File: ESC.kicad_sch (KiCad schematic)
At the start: 23 parts, among them IC1 DRV8302DCA, J1 Prog, J2 Conn_01x01, J3 Conn_01x01, J4 Conn_01x01, J5 Conn_ALIM_MOTOR, J6 Conn_ALIM_AUX, Q1 2N7002, U1 ATmega328P-AU_full, Y1 CSTCE

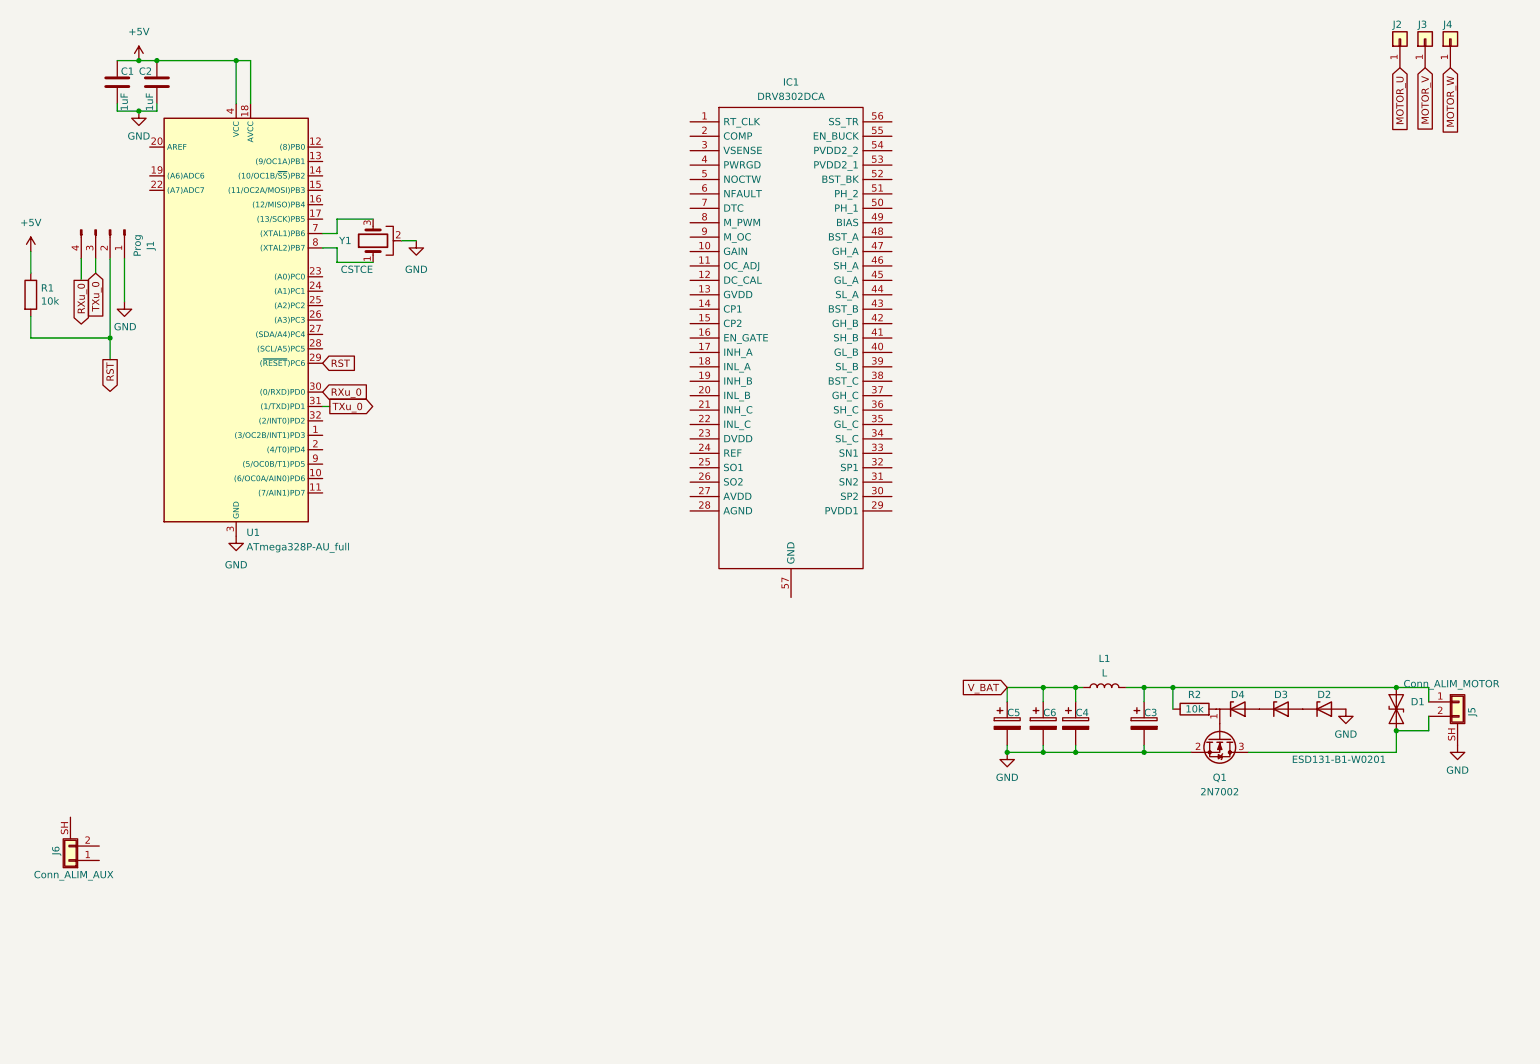
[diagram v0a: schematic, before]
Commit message: aa
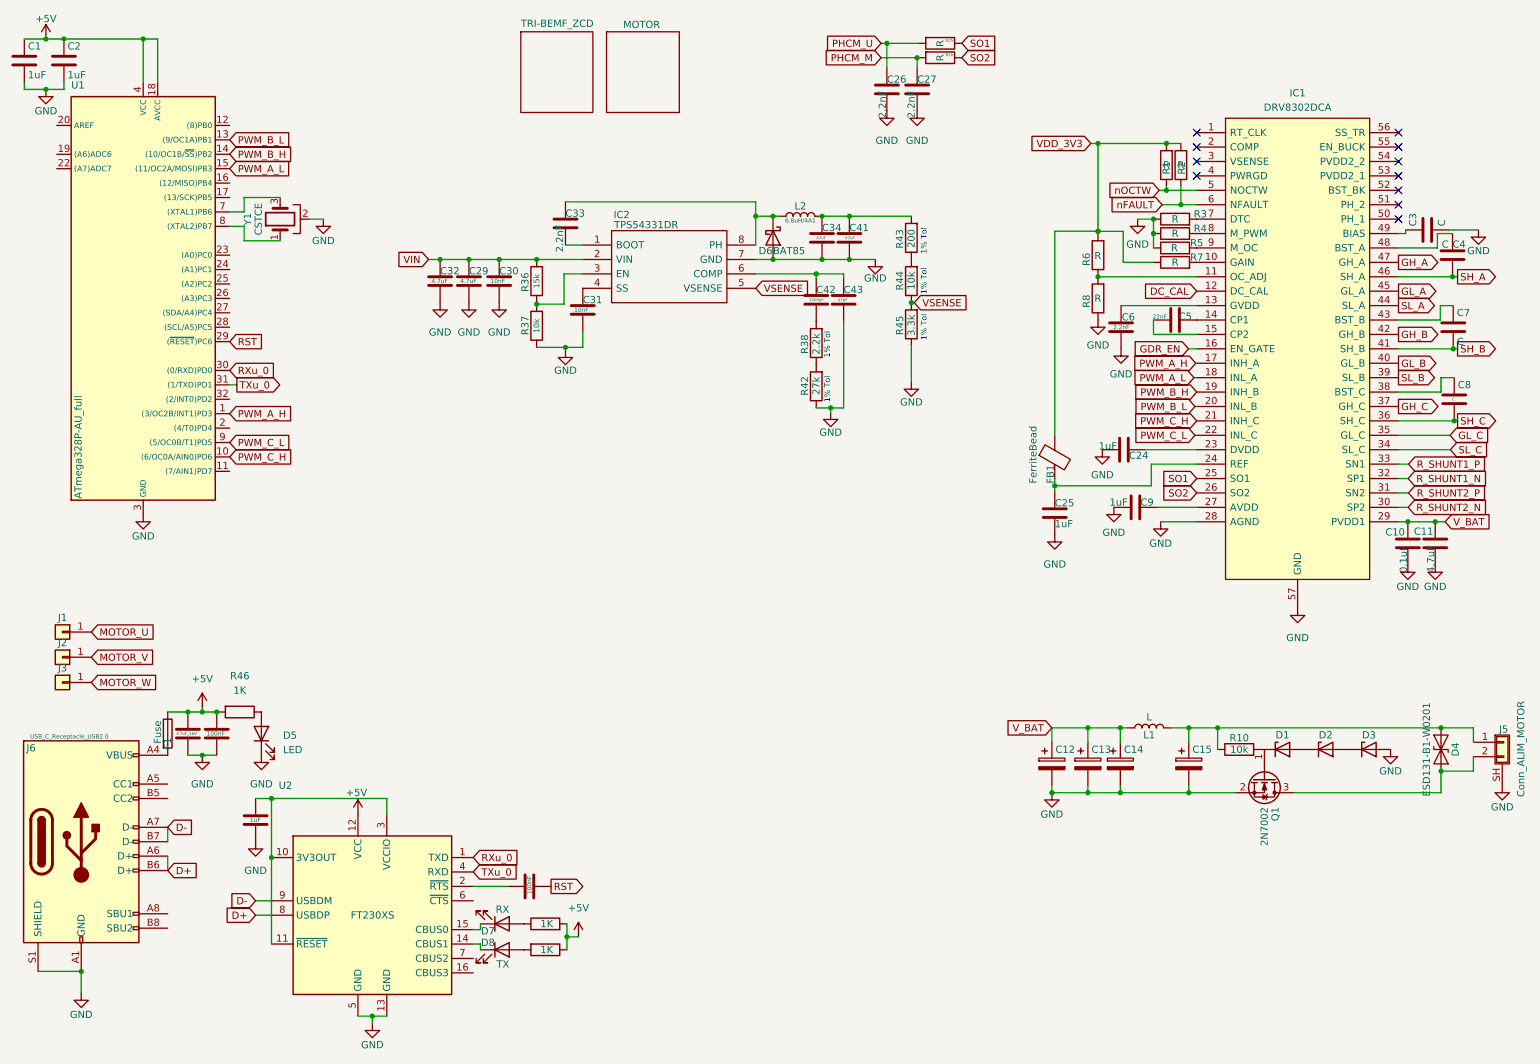
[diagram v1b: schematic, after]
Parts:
- removed J1: Prog, Connector_PinHeader_2.54mm:PinHeader_1x04_P2.54mm_Vertical, symbol etuve-rescue:Conn_01x04_Male-Connector
- removed J6: Conn_ALIM_AUX, symbol Connector_Generic_Shielded:Conn_01x02_Shielded
- added 6.8uH/4A1: L2, Inductor_SMD:L_1206_3216Metric, symbol Device:L
- added C10: 0.1uF, Capacitor_SMD:C_1206_3216Metric, symbol Device:C
- added C11, C29, C32: 4.7uF, Capacitor_SMD:C_1206_3216Metric, symbol Device:C
- added C24, C25, C9: 1uF, Capacitor_SMD:C_1206_3216Metric, symbol Device:C
- added C26, C27, C33, C6: 2.2nF, Capacitor_SMD:C_1206_3216Metric, symbol Device:C
- added C3, C4, C7, C8: C, Capacitor_SMD:C_1206_3216Metric, symbol Device:C
- added C30, C31: 10nF, Capacitor_SMD:C_1206_3216Metric, symbol Device:C
- added C34, C41: 47uF, Capacitor_SMD:C_1206_3216Metric, symbol Device:C
- added C42: 1000pF, Capacitor_SMD:C_1206_3216Metric, symbol Device:C
- added C43: 47pF, Capacitor_SMD:C_1206_3216Metric, symbol Device:C
- added C44: 1uF, Capacitor_SMD:C_1206_3216Metric_Pad1.33x1.80mm_HandSolder, symbol Device:C
- added C45: 4.7uF_16V, Capacitor_SMD:C_1206_3216Metric_Pad1.33x1.80mm_HandSolder, symbol Device:C
- added C46, C47: 100nF, Capacitor_SMD:C_1206_3216Metric_Pad1.33x1.80mm_HandSolder, symbol Device:C
- added C5: 22nF, Capacitor_SMD:C_1206_3216Metric, symbol Device:C
- added D5: LED, LED_SMD:LED_1206_3216Metric_Pad1.42x1.75mm_HandSolder, symbol Device:LED
- added D6: BAT85, Diode_THT:D_DO-35_SOD27_P7.62mm_Horizontal, symbol Diode:BAT85
- added D7: RX, LED_SMD:LED_1206_3216Metric_Pad1.42x1.75mm_HandSolder, symbol Device:LED
- added D8: TX, LED_SMD:LED_1206_3216Metric_Pad1.42x1.75mm_HandSolder, symbol Device:LED
- added F1: Fuse, Fuse:Fuse_1206_3216Metric_Pad1.42x1.75mm_HandSolder, symbol Device:Fuse
- added FB1: FerriteBead, symbol Device:FerriteBead
- added IC2: TPS54331DR, SOIC127P600X175-8N, symbol Dam_libkicad:TPS54331DR
- added J6: USB_C_Receptacle_USB2.0, Connector_USB:USB_C_Receptacle_GCT_USB4105-xx-A_16P_TopMnt_Horizontal, symbol Connector:USB_C_Receptacle_USB2.0
- added R2, R25, R26, R3, R4, R5, R6, R7, R8: R, Resistor_SMD:R_1206_3216Metric, symbol Device:R
- added R36: 15k, Resistor_SMD:R_1206_3216Metric, symbol Device:R
- added R37, R44: 10k, Resistor_SMD:R_1206_3216Metric, symbol Device:R
- added R38: 2.2k, Resistor_SMD:R_1206_3216Metric, symbol Device:R
- added R42: 27k, Resistor_SMD:R_1206_3216Metric, symbol Device:R
- added R43: 200, Resistor_SMD:R_1206_3216Metric, symbol Device:R
- added R45: 3.3k, Resistor_SMD:R_1206_3216Metric, symbol Device:R
- added R46, R47, R48: 1K, Resistor_SMD:R_1206_3216Metric_Pad1.30x1.75mm_HandSolder, symbol Device:R
- added U2: FT230XS, Package_SO:SSOP-16_5.3x6.2mm_P0.65mm, symbol Interface_USB:FT230XS
- C12: renamed from C5; footprint (none) -> Capacitor_SMD:CP_Elec_4x3
- C13: renamed from C6; footprint (none) -> Capacitor_SMD:CP_Elec_4x3
- C14: renamed from C4; footprint (none) -> Capacitor_SMD:CP_Elec_4x3
- C15: renamed from C3; footprint (none) -> Capacitor_SMD:CP_Elec_4x3
- IC1: footprint SOP50P810X120-57N -> Dam_libkicad:SOP50P810X120-57N
- L1: footprint (none) -> Inductor_SMD:L_1206_3216Metric
- R1: value 10k -> R; footprint Dam_libkicad:1206 -> Resistor_SMD:R_1206_3216Metric
- R10: renamed from R2; footprint (none) -> Resistor_SMD:R_1206_3216Metric
- renumbered D4 to D1, D3 to D2, D2 to D3, D1 to D4, J2 to J1, J3 to J2, J4 to J3
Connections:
- net +5V: now also C45.1, C46.1, F1.1, R46.2, R47.2, R48.1, U2.12 (VCC); no longer R1.1
- net GND: now also IC1.28 (AGND), IC1.57 (GND), C10.2, C11.2, C24.2, C25.2, C26.2, C27.2, C29.2, C3.2, C30.2, C31.2, C32.2, C34.2, C41.2, C43.2, C44.1, C45.2, C46.2, C6.2, C9.2, D5.1 (K), D6.2 (A), IC2.7 (GND), J6.A1 (GND), J6.A12 (GND), J6.B1 (GND), J6.B12 (GND), J6.S1 (SHIELD), R3.1, R37.1, R4.1, R42.1, R45.1, R5.1, R8.1, U2.13 (GND), U2.5 (GND)
- net RST: now also C47.1; no longer R1.2
- net RXu_0: now also U2.1 (TXD)
- net TXu_0: now also U2.4 (RXD)
- net V_BAT: now also IC1.29 (PVDD1), C10.1, C11.1
- net at IC1.10 (GAIN): now also R7.2
- net at IC1.11 (OC_ADJ): now also R6.1, R8.2
- net DC_CAL: now reaches IC1.12 (DC_CAL)
- net at IC1.13 (GVDD): now also C6.1
- net at IC1.14 (CP1): now also C5.1
- net at IC1.15 (CP2): now also C5.2
- net GDR_EN: now reaches IC1.16 (EN_GATE)
- net PWM_A_H: now reaches IC1.17 (INH_A)
- net PWM_A_H: now also U1.1 ((3/OC2B/INT1)PD3)
- net PWM_A_L: now reaches IC1.18 (INL_A)
- net PWM_A_L: now also U1.15 ((11/OC2A/MOSI)PB3)
- net PWM_B_H: now reaches IC1.19 (INH_B)
- net PWM_B_H: now also U1.14 ((10/OC1B/~{SS})PB2)
- net PWM_B_L: now reaches IC1.20 (INL_B)
- net PWM_B_L: now also U1.13 ((9/OC1A)PB1)
- net PWM_C_H: now reaches IC1.21 (INH_C)
- net PWM_C_H: now also U1.10 ((6/OC0A/AIN0)PD6)
- net PWM_C_L: now reaches IC1.22 (INL_C)
- net PWM_C_L: now also U1.9 ((5/OC0B/T1)PD5)
- net at IC1.23 (DVDD): now also C24.1
- net at IC1.24 (REF): now also C25.1, FB1.2
- net SO1: now reaches IC1.25 (SO1)
- net SO1: now also R25.1
- net SO2: now reaches IC1.26 (SO2)
- net SO2: now also R26.1
- net at IC1.27 (AVDD): now also C9.1
- net R_SHUNT2_N: now reaches IC1.30 (SP2)
- net R_SHUNT2_P: now reaches IC1.31 (SN2)
- net R_SHUNT1_N: now reaches IC1.32 (SP1)
- net R_SHUNT1_P: now reaches IC1.33 (SN1)
- net SL_C: now reaches IC1.34 (SL_C)
- net GL_C: now reaches IC1.35 (GL_C)
- net SH_C: now reaches IC1.36 (SH_C)
- net SH_C: now also C8.2
- net GH_C: now reaches IC1.37 (GH_C)
- net at IC1.38 (BST_C): now also C8.1
- net SL_B: now reaches IC1.39 (SL_B)
- net GL_B: now reaches IC1.40 (GL_B)
- net SH_B: now reaches IC1.41 (SH_B)
- net SH_B: now also C7.2
- net GH_B: now reaches IC1.42 (GH_B)
- net at IC1.43 (BST_B): now also C7.1
- net SL_A: now reaches IC1.44 (SL_A)
- net GL_A: now reaches IC1.45 (GL_A)
- net SH_A: now reaches IC1.46 (SH_A)
- net SH_A: now also C4.2
- net GH_A: now reaches IC1.47 (GH_A)
- net at IC1.48 (BST_A): now also C4.1
- net at IC1.49 (BIAS): now also C3.1
- net nOCTW: now reaches IC1.5 (NOCTW)
- net nOCTW: now also R1.1
- net nFAULT: now reaches IC1.6 (NFAULT)
- net nFAULT: now also R2.1
- net at IC1.7 (DTC): now also R3.2
- net at IC1.8 (M_PWM): now also R4.2
- net at IC1.9 (M_OC): now also R5.2
- new net: 6.8uH/4A1.2, C34.1, C41.1, R43.2
- new net: D7.1 (K), U2.15 (CBUS0)
- new net: D7.2 (A), R47.1
- new net: R38.1, R42.2
- new net: 6.8uH/4A1.1, C33.1, D6.1 (K), IC2.8 (PH)
- new net: C33.2, IC2.1 (BOOT)
- new net: IC2.3 (EN), R36.1, R37.2
- new net: C31.1, IC2.4 (SS)
- new net: C42.1, C43.1, IC2.6 (COMP)
- new net: C47.2, U2.2 (~{RTS})
- new net: F1.2, J6.A4 (VBUS), J6.A9 (VBUS), J6.B4 (VBUS), J6.B9 (VBUS)
- new net: R43.1, R44.2
- new net: C44.2, U2.10 (3V3OUT), U2.11 (~{RESET}), U2.3 (VCCIO)
- new net: C42.2, R38.2
- new net: D8.1 (K), U2.14 (CBUS1)
- new net: D8.2 (A), R48.2
- new net: D5.2 (A), R46.1
- new net D+: J6.A6 (D+), J6.B6 (D+), U2.8 (USBDP)
- new net D-: J6.A7 (D-), J6.B7 (D-), U2.9 (USBDM)
- new net PHCM_M: C27.1, R26.2
- new net PHCM_U: C26.1, R25.2
- new net VDD_3V3: FB1.1, R1.2, R2.2, R6.2, R7.1
- new net VIN: C29.1, C30.1, C32.1, IC2.2 (VIN), R36.2
- new net VSENSE: IC2.5 (VSENSE), R44.1, R45.2
- no-connect marks 0 -> 11
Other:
- added sheet MOTOR (untitled.kicad_sch)
- added sheet TRI-BEMF_ZCD (TRI-BEMF_ZCD.kicad_sch)
- note added: "1% Tol"
- moved on the sheet: C1, C12, C13, C14, C15, C2, D1, D2, D3, D4, J1, J2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

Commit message: v0.02
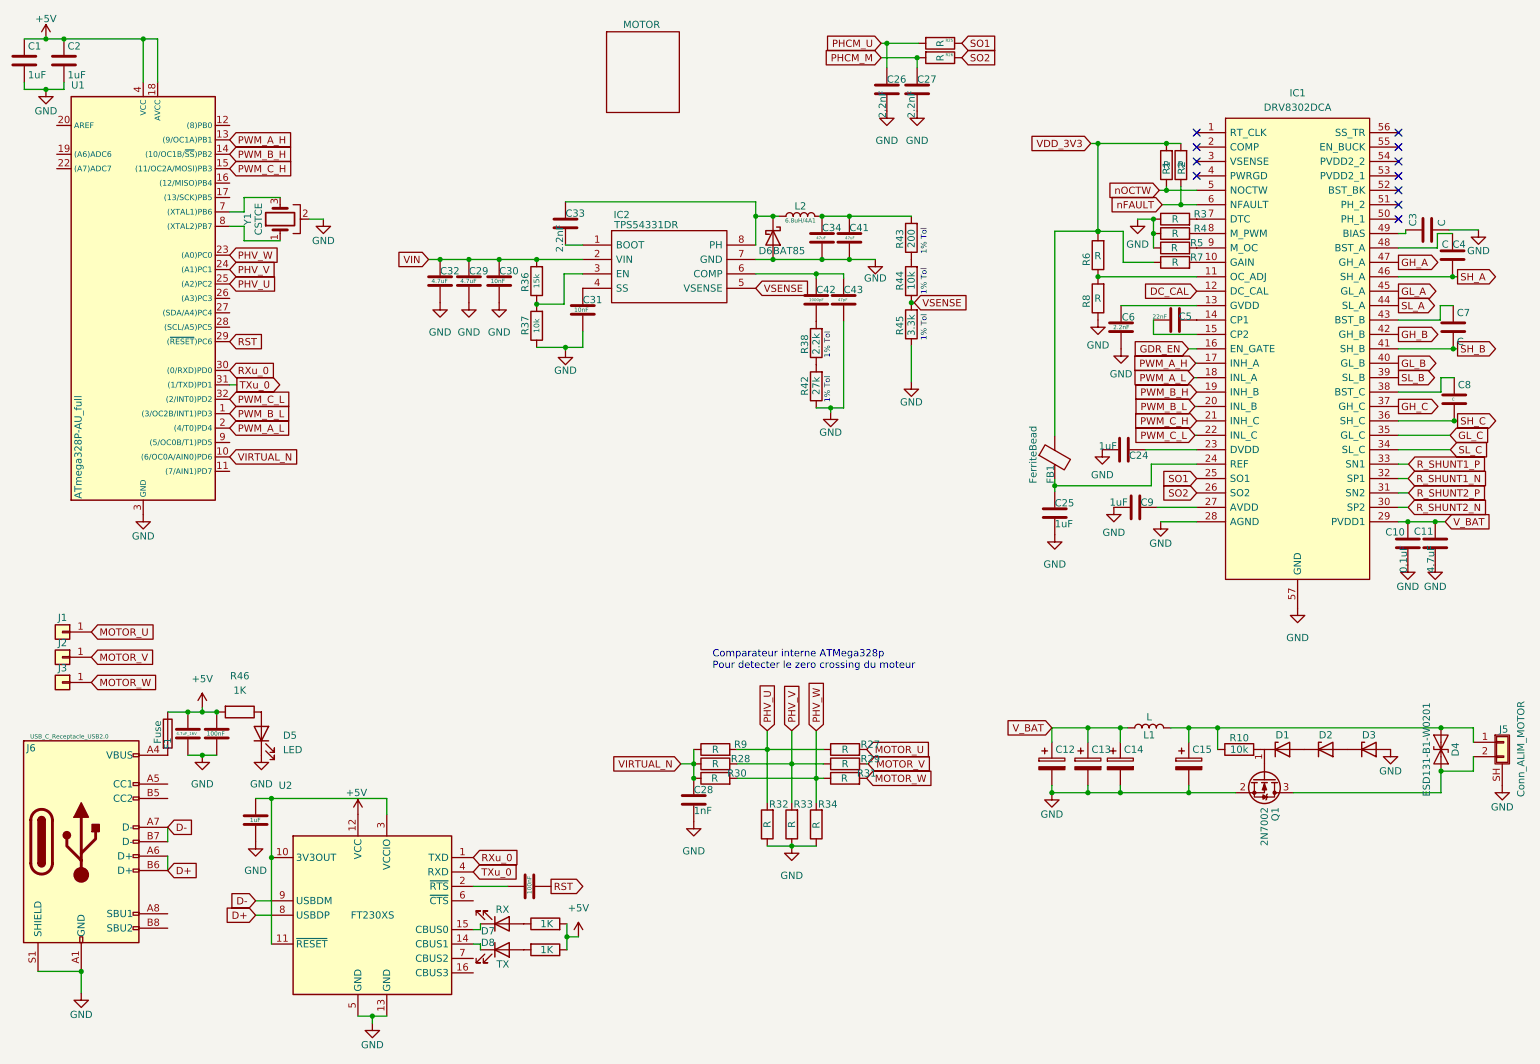
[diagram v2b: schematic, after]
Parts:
- added C28: 1nF, Capacitor_SMD:C_1206_3216Metric, symbol Device:C
- added R27, R28, R29, R30, R31, R32, R33, R34, R9: R, Resistor_SMD:R_1206_3216Metric, symbol Device:R
- FB1: footprint (none) -> Inductor_SMD:L_1206_3216Metric
- IC2: footprint SOIC127P600X175-8N -> Dam_libkicad:SOIC127P600X175-8N
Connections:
- net GND: now also C28.2, R32.1, R33.1, R34.1
- net MOTOR_U: now also R27.2
- net MOTOR_V: now also R29.2
- net MOTOR_W: now also R31.2
- net PWM_A_H: now also U1.13 ((9/OC1A)PB1); no longer U1.1 ((3/OC2B/INT1)PD3)
- net PWM_A_L: now also U1.2 ((4/T0)PD4); no longer U1.15 ((11/OC2A/MOSI)PB3)
- net PWM_B_L: now also U1.1 ((3/OC2B/INT1)PD3); no longer U1.13 ((9/OC1A)PB1)
- net PWM_C_H: now also U1.15 ((11/OC2A/MOSI)PB3); no longer U1.10 ((6/OC0A/AIN0)PD6)
- net PWM_C_L: now also U1.32 ((2/INT0)PD2); no longer U1.9 ((5/OC0B/T1)PD5)
- net PHV_W: now reaches U1.23 ((A0)PC0)
- net PHV_W: now also R30.2, R31.1, R34.2
- net PHV_V: now reaches U1.24 ((A1)PC1)
- net PHV_V: now also R28.2, R29.1, R33.2
- net PHV_U: now reaches U1.25 ((A2)PC2)
- net PHV_U: now also R27.1, R32.2, R9.2
- new net VIRTUAL_N: C28.1, R28.1, R30.1, R9.1, U1.10 ((6/OC0A/AIN0)PD6)
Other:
- removed sheet TRI-BEMF_ZCD
- note added: "Comparateur interne ATMega328p Pour detecter le zero crossing du moteur"
